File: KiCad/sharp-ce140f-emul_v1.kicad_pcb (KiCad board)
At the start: 2 copper layers, 34.5 x 61.2 mm, 42 parts, among them J2 Micro_SD_Card_Det, J3 Conn_01x15, J4 Conn_01x15, J5 Conn_01x01, J6 Conn_01x01, J7 Conn_01x01, J8 Sharp PC 11-pin, J9 Conn_01x01, Q2 BSS138, Q3 BSS138, Q4 BSS138, Q5 BSS138, Q6 BSS138, U3 NUCLEO-L432KC

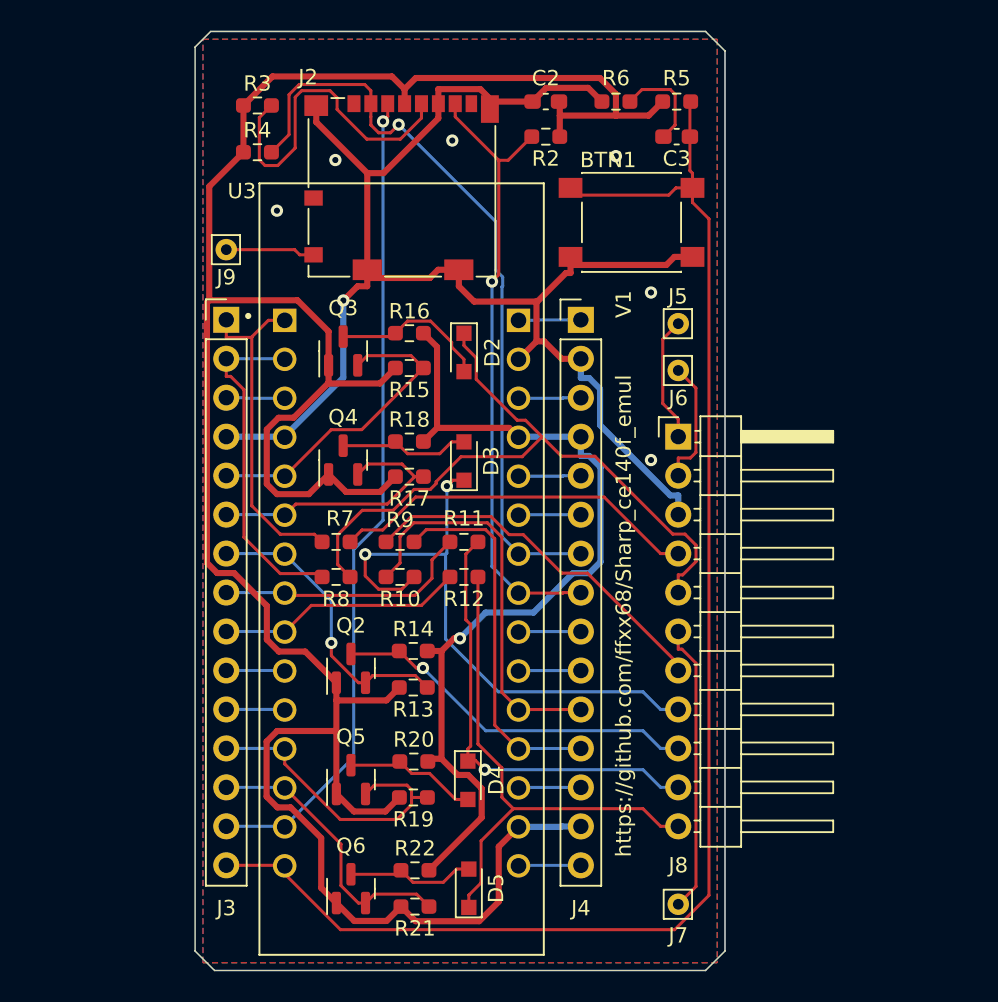
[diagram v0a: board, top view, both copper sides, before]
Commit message: Final review before PCB manufacturing
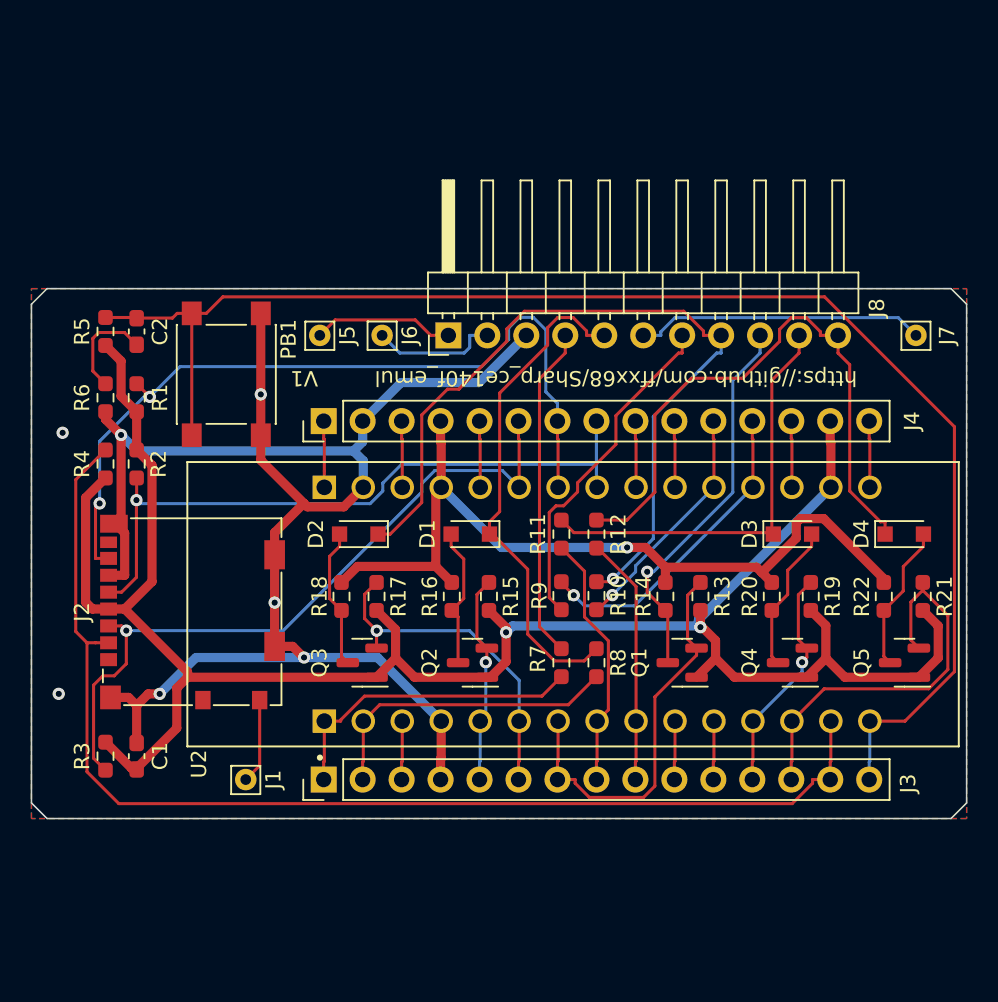
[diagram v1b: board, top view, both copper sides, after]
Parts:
- removed BTN1: User_button, Button_Switch_SMD:SW_Push_1P1T_NO_6x6mm_H9.5mm
- removed C3: 100n, Capacitor_SMD:C_0603_1608Metric_Pad1.08x0.95mm_HandSolder
- removed D5: 1N4148, Diode_SMD:D_SOD-323_HandSoldering
- removed J9: Conn_01x01, Connector_Pin:Pin_D0.7mm_L6.5mm_W1.8mm_FlatFork
- removed Q6: BSS138, Package_TO_SOT_SMD:SOT-23
- removed U3: NUCLEO-L432KC, MyLibrary:MODULE_NUCLEO-L432KC
- added C1: 100n, Capacitor_SMD:C_0603_1608Metric_Pad1.08x0.95mm_HandSolder, F.Cu at (156.2, 147.3)
- added D1: 1N4148, Diode_SMD:D_SOD-323_HandSoldering, F.Cu at (178.0, 132.8)
- added J1: Conn_01x01, Connector_Pin:Pin_D0.7mm_L6.5mm_W1.8mm_FlatFork, F.Cu at (163.3, 148.8)
- added PB1: User_button, Button_Switch_SMD:SW_Push_1P1T_NO_6x6mm_H9.5mm, F.Cu at (162.1, 122.4)
- added Q1: BSS138, Package_TO_SOT_SMD:SOT-23, F.Cu at (191.8, 141.2)
- added R1: 47k, Resistor_SMD:R_0603_1608Metric_Pad0.98x0.95mm_HandSolder, F.Cu at (156.2, 124.0)
- added U2: NUCLEO-L432KC, MyLibrary:MODULE_NUCLEO-L432KC, F.Cu at (184.7, 137.4)
- moved R3 43.6 mm to (154.2, 147.3), turned to -90 degrees
- moved J7 40.2 mm to (207.0, 119.9), turned to 90 degrees
- moved R5 40.1 mm to (154.2, 119.6), turned to -90 degrees
- moved R21 38.8 mm to (207.5, 136.9), turned to -90 degrees
- moved R6 38.5 mm to (154.2, 124.0), turned to 90 degrees
- moved Q5 36.9 mm to (206.3, 141.2), turned to 180 degrees
- moved R22 35.4 mm to (204.9, 136.9), turned to 90 degrees
- moved R2 34.2 mm to (156.2, 128.3), turned to -90 degrees
- moved D4 32.7 mm to (206.2, 132.8), turned to 0 degrees
- moved Q4 32.1 mm to (199.0, 141.2), turned to 180 degrees
- moved J2 30.9 mm to (159.8, 137.9), turned to 90 degrees
- moved J3 30.6 mm to (168.4, 148.8), turned to 90 degrees
- moved C2 30.6 mm to (156.2, 119.6), turned to -90 degrees
- moved R19 29.0 mm to (200.2, 136.9), turned to -90 degrees
- moved R20 25.7 mm to (197.6, 136.9), turned to 90 degrees
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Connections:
- C2 pad 1: +3V3 -> CN3_15
- C2 pad 2: GND -> /rc_btn
- D2 pad 1: /conn_dout -> /conn_din
- D2 pad 2: /Level Conv2/conv_HV -> /Level Conv3/conv_HV
- D3 pad 1: /conn_din -> /conn_sel2
- D3 pad 2: /Level Conv3/conv_HV -> /Level Conv4/conv_HV
- D4 pad 1: /conn_sel2 -> /conn_sel1
- D4 pad 2: /Level Conv4/conv_HV -> /Level Conv5/conv_HV
- J2 pad 2: CN4_7 -> CN3_14
- J2 pad 3: CN3_14 -> CN4_6
- J2 pad 5: /sd_sck -> CN4_8
- J2 pad 7: CN4_8 -> CN4_7
- Q2 pad 2: CN3_7 -> CN3_5
- Q2 pad 3: /conn_ack -> /Level Conv2/conv_HV
- Q3 pad 2: CN3_5 -> CN3_6
- Q3 pad 3: /Level Conv2/conv_HV -> /Level Conv3/conv_HV
- Q4 pad 2: CN3_6 -> CN3_12
- Q4 pad 3: /Level Conv3/conv_HV -> /Level Conv4/conv_HV
- Q5 pad 2: CN3_12 -> CN3_13
- Q5 pad 3: /Level Conv4/conv_HV -> /Level Conv5/conv_HV
- R3 pad 2: /sd_sck -> CN4_6
- R4 pad 2: CN4_7 -> CN3_14
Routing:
- net CN4_6: track 4.08 -> 47.1 mm, vias 0 -> 1
- net +3V3: track 173.6 -> 135.2 mm, vias 0 -> 2
- net CN3_14: track 53.7 -> 77.4 mm, vias 1 -> 0
- net /sd_sck: track 21.8 -> 0.00 mm
- net /conn_din: track 38.9 -> 53.2 mm, vias 2 -> 1
- net /conn_dout: track 45.0 -> 32.9 mm
- net GND: track 95.7 -> 107.5 mm
- net CN4_11: track 26.2 -> 15.5 mm, vias 0 -> 1
- net CN3_13: track 18.5 -> 26.1 mm
- net CN3_5: track 20.7 -> 13.6 mm, vias 0 -> 1
- net CN3_7: track 19.2 -> 26.1 mm, vias 1 -> 0
- net CN3_12: track 20.3 -> 14.9 mm, vias 0 -> 1
- net /conn_sel1: track 34.9 -> 39.6 mm
- net CN3_6: track 18.2 -> 22.0 mm, vias 0 -> 1
- net CN4_7: track 49.8 -> 53.6 mm, vias 1 -> 2
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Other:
- board size 34.5 x 61.2 mm -> 61 x 34.5 mm
